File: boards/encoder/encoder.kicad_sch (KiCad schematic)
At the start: 36 parts, among them J1 Conn_PWR, J2 SWD, J3 Sensore, J4 Sensore, SW1 SW_SPST, SW2 SW_SPST, SW3 SW_Push, U1 MSPM0G310x, U2 TPS62A02A, U9 M24C08

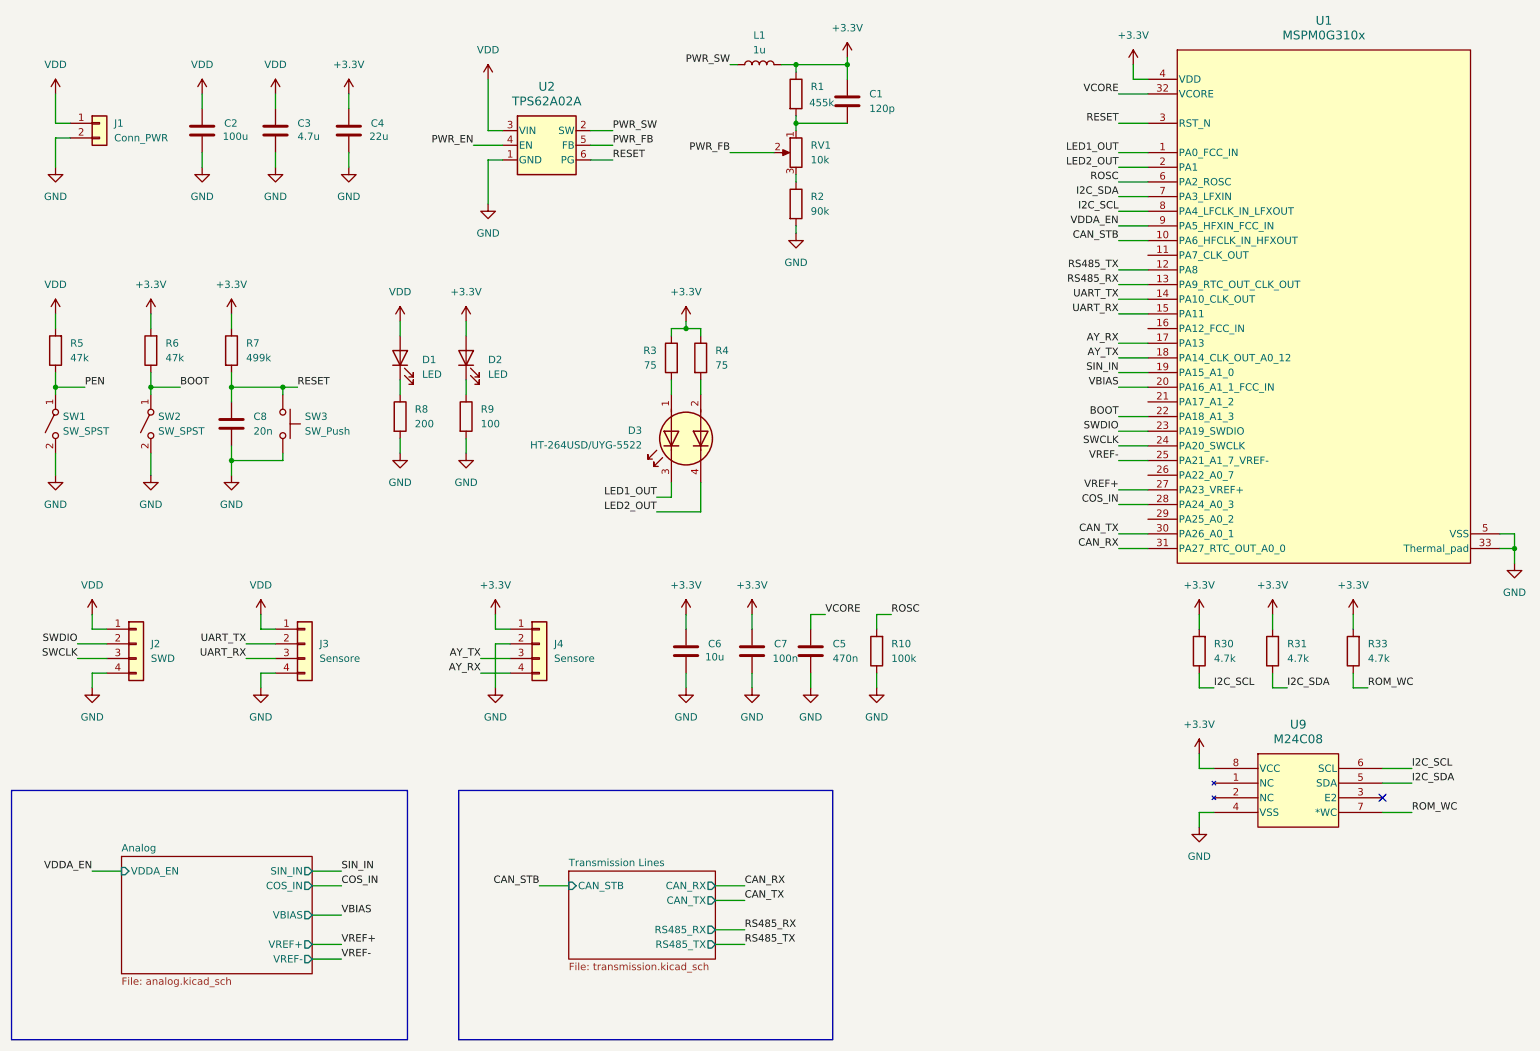
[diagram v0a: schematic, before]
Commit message: v0.1.17
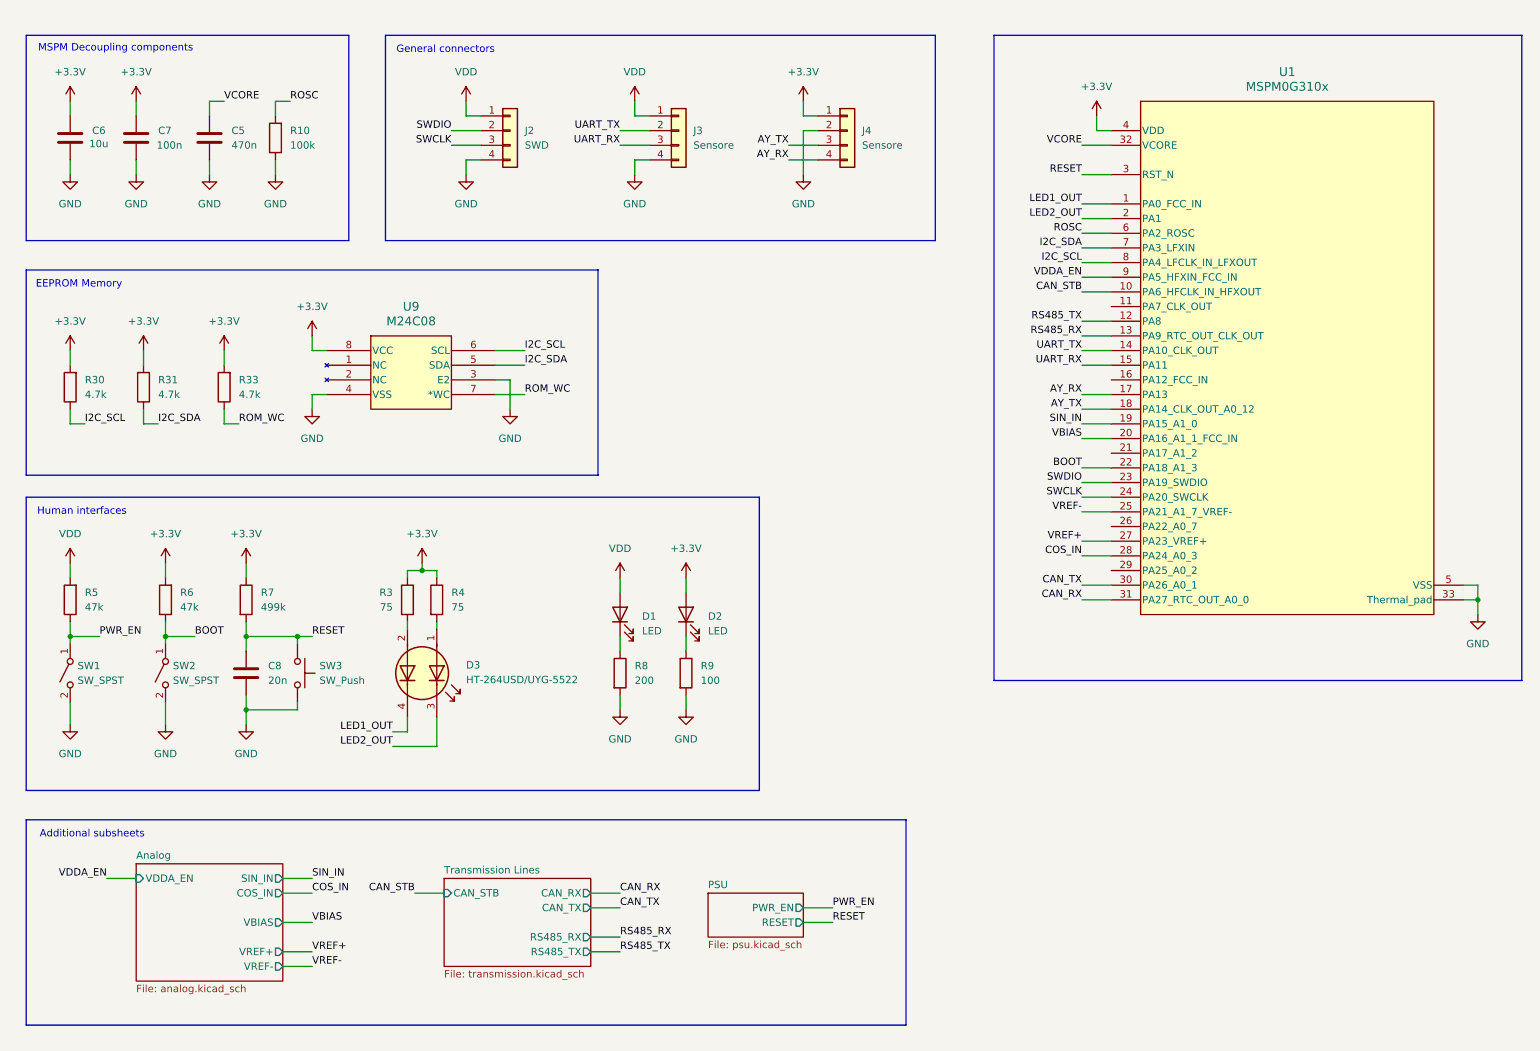
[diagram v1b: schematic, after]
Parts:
- removed C1: 120p, symbol Device:C
- removed C2: 100u, symbol Device:C
- removed C3: 4.7u, symbol Device:C
- removed C4: 22u, symbol Device:C
- removed J1: Conn_PWR, symbol Connector_Generic:Conn_01x02
- removed L1: 1u, symbol Device:L
- removed R1: 455k, symbol Device:R
- removed R2: 90k, symbol Device:R
- removed RV1: 10k, symbol Device:R_Potentiometer
- removed U2: TPS62A02A, SOT6_DRL_TEX, symbol Regulator_Switching:TPS62A02A
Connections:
- net PEN is gone; now on net PWR_EN: R5.1, SW1.1 (A)
- net GND: now also U9.3 (E2)
- net LED1_OUT: now also D3.4 (K2); no longer D3.3 (K1)
- net LED2_OUT: now also D3.3 (K1); no longer D3.4 (K2)
- net at D3.1 (A1): now also R4.2; no longer R3.2
- net at D3.2 (A2): now also R3.2; no longer R4.2
- no-connect marks 1 -> 0
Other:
- added sheet PSU (psu.kicad_sch)
- note added: "Additional subsheets"
- note added: "EEPROM Memory"
- note added: "General connectors"
- note added: "Human interfaces"
- note added: "MSPM Decoupling components"
- moved on the sheet: C5, C6, C7, C8, D1, D2, D3, J2, J3, J4, R10, R3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
